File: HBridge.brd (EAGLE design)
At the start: 59.7 x 53.3 mm, 40 parts, among them IC1 74HC08D, IC2 A4954, SW1 SWITCH-DP3T, SW2 SWITCH-DP3T

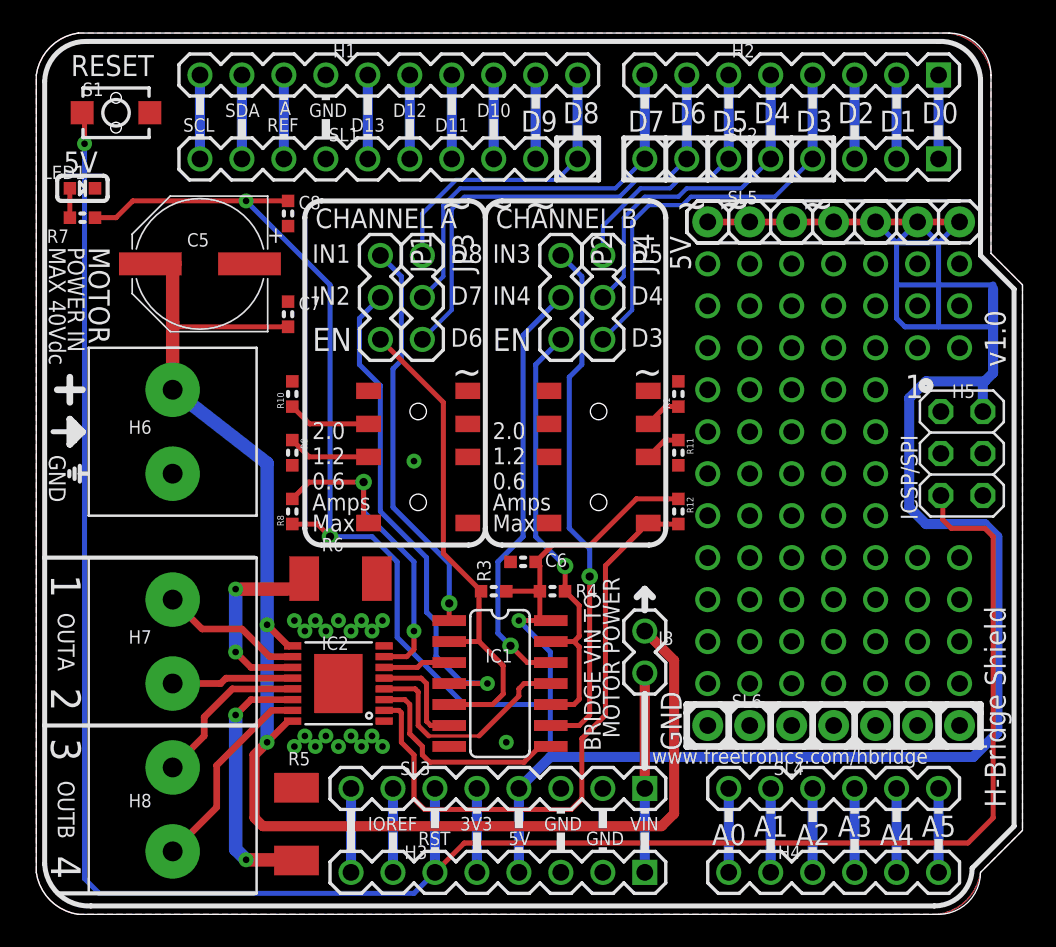
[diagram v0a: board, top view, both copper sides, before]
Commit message: Annotation updates for release
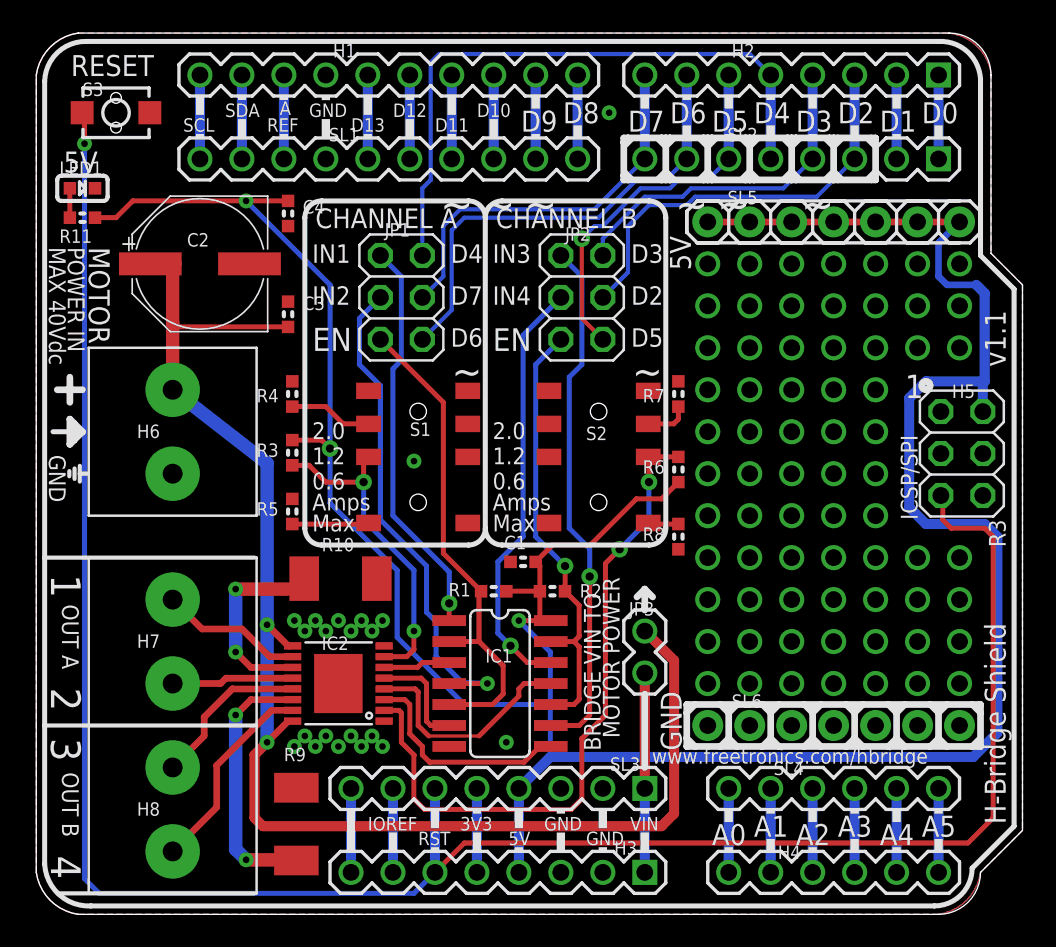
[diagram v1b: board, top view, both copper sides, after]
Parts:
- removed J3: (no value), freetronics-master-v1:1X02
- removed JP4: (no value), freetronics-master-v1.1:1X03
- removed R12: 2K2, freetronics-master-v1:0603
- removed SW1: SWITCH-DP3T, freetronics-jon:MS-23C01
- added R2: 10K 0603, freetronics-master-v1:0603
- added S3: RESET, freetronics-master-v1:TACTILE_SWITCH_SMD_2PIN_TINY
- C1, C4: value 100nF -> 100nF 0603
- C2: value 100uF -> 100uF 50V
- C3: value 220nF -> 220nF 50V 0603
- IC1: value 74HC08D -> 74HC08D SOIC-14
- IC2: value A4954 -> A4954 TSSOP-16
- JP1, JP2: device freetronics-master-v1.1:1X03 -> freetronics-master-v1:2X03
- JP3: device freetronics-master-v1.1:1X03 -> freetronics-master-v1:1X02
- R1: value 3K3 -> 10K 0603
- R10: value 3K3 -> 0.25R 1W 2010; device freetronics-master-v1:0603 -> rcl:R2010
- R11: value 953R -> 2K2 0603; device freetronics-master-v1:0603 -> freetronics:0603
- R3: value 10K -> 2K2 0603
- R4: value 10K -> 3K3 1% 0603
- R5: value 0.25R 1W -> 953R 1% 0603; device rcl:R2010 -> freetronics-master-v1:0603
- R6: value 0.25R 1W -> 2K2 0603; device rcl:R2010 -> freetronics-master-v1:0603
- R7: value 2K2 -> 3K3 1% 0603; device freetronics:0603 -> freetronics-master-v1:0603
- R8: value 2K2 -> 953R 1% 0603
- R9: value 953R -> 0.25R 1W 2010; device freetronics-master-v1:0603 -> rcl:R2010
- S1: value RESET -> SWITCH-DP3T MS-23C01; device freetronics-master-v1:TACTILE_SWITCH_SMD_2PIN_TINY -> freetronics-jon:MS-23C01
- S2: value SWITCH-DP3T -> SWITCH-DP3T MS-23C01
- moved R11 38.8 mm to (2.79, 42.2), turned to 180 degrees
- moved R7 37.6 mm to (38.9, 31.5), turned to 90 degrees
- moved JP3 28.6 mm to (36.8, 14.6), turned to 90 degrees
- moved S1 27.7 mm to (23.1, 27.7)
- moved R8 23.4 mm to (38.9, 22.9), turned to 270 degrees
- moved R9 22.5 mm to (15.7, 5.46)
- moved R6 21.5 mm to (38.9, 26.9), turned to 90 degrees
- moved R4 19.8 mm to (15.5, 31.5), turned to 90 degrees
- moved R5 18.9 mm to (15.5, 24.4), turned to 90 degrees
- moved R1 16.4 mm to (27.7, 19.6), turned to 180 degrees
- moved R3 14.8 mm to (15.5, 27.9), turned to 270 degrees
- moved R10 11.6 mm to (18.4, 20.3), turned to 180 degrees
- moved JP2 2.84 mm to (33.0, 37.3)
- moved JP1 2.84 mm to (22.1, 37.3)
- renumbered C5 to C2, C6 to C1, C7 to C3, C8 to C4, SW2 to S2
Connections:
- net +5V: now also R1.1, R11.1, R2.2, R6.1; no longer R12.1, R4.2, R7.1, R8.1
- net D2: now also JP2.4
- net D3: now also JP2.2; no longer JP4.3
- net D4: now also JP1.2; no longer JP4.2
- net D5: now also JP2.6; no longer JP4.1
- net D6: now also JP1.6; no longer JP3.3
- net D7: now also JP1.4; no longer JP3.2
- net D8: no longer JP3.1
- net EN-A: now also JP1.5, R1.2; no longer JP1.3, R3.2
- net EN-B: now also JP2.5, R2.1; no longer JP2.3, R4.1
- net GND: now also R10.1, R4.2, R5.2, R7.2, R8.2, R9.1, S3.2; no longer R1.2, R10.2, R11.2, R5.1, R6.1, R9.2, S1.2
- net IN2: now also JP1.3; no longer JP1.2
- net IN4: now also JP2.3; no longer JP2.2
- net N$13: now also R9.2; no longer R5.2
- net N$14: now also R10.2; no longer R6.2
- net N$15: now also R4.1, S1.1-2; no longer R10.1, SW1.1-2
- net N$21: now also R5.1, S1.1-3; no longer R9.1, SW1.1-3
- net N$22: now also R11.2; no longer R7.2
- net N$4: now also R8.1; no longer R11.1
- net N$49: now also R7.1; no longer R1.1
- net RESET: now also S3.1; no longer S1.1
- net VBB: now also JP3.2; no longer J3.2
- net VIN: now also JP3.1; no longer J3.1
- net VREF12: now also R3.2, S1.1-C; no longer R8.2, SW1.1-C
- net VREF34: now also R6.2; no longer R12.2
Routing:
- net +5V: track 203.6 -> 177.5 mm
- net D2: track 5.08 -> 25.4 mm
- net D4: track 20.8 -> 38.3 mm
- net D8: track 18.4 -> 5.08 mm
- net D5: track 16.2 -> 22.6 mm, vias 0 -> 1
- net D3: track 25.4 -> 20.8 mm
- net VREF34: track 37.5 -> 41.5 mm, vias 0 -> 2
- net VREF12: track 20.7 -> 19.8 mm
- net D7: track 24.5 -> 23.8 mm
- net D6: track 29.2 -> 28.4 mm
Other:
- board text added: "(c) 2013 Freetronics Pty Ltd"
- board text added: "H-Bridge Motor Controller Shield"
- board text added: "K"
- board text added: "OUT A"
- board text added: "OUT B"
- board text added: "R3"
- board text added: "S2"
- board text added: "S3"
- board text added: "V1.1"
- board text added: "v1.1"
- board text removed: "(c) 2012 Freetronics Pty Ltd"
- board text removed: "H-Bridge Motor Controller"
- board text removed: "OUTA"
- board text removed: "OUTB"
- board text removed: "V1.0"
- board text removed: "v1.0"
